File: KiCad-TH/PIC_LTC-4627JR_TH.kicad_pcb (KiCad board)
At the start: 2 copper layers, 43.2 x 48.3 mm, 17 parts, among them J1 Conn_01x05_Male, J2 Conn_01x04, Q1 Q_NPN_EBC, Q2 Q_NPN_EBC, Q3 Q_NPN_EBC, Q4 Q_NPN_EBC, Q5 Q_NPN_EBC, U1 PIC16F18344-P

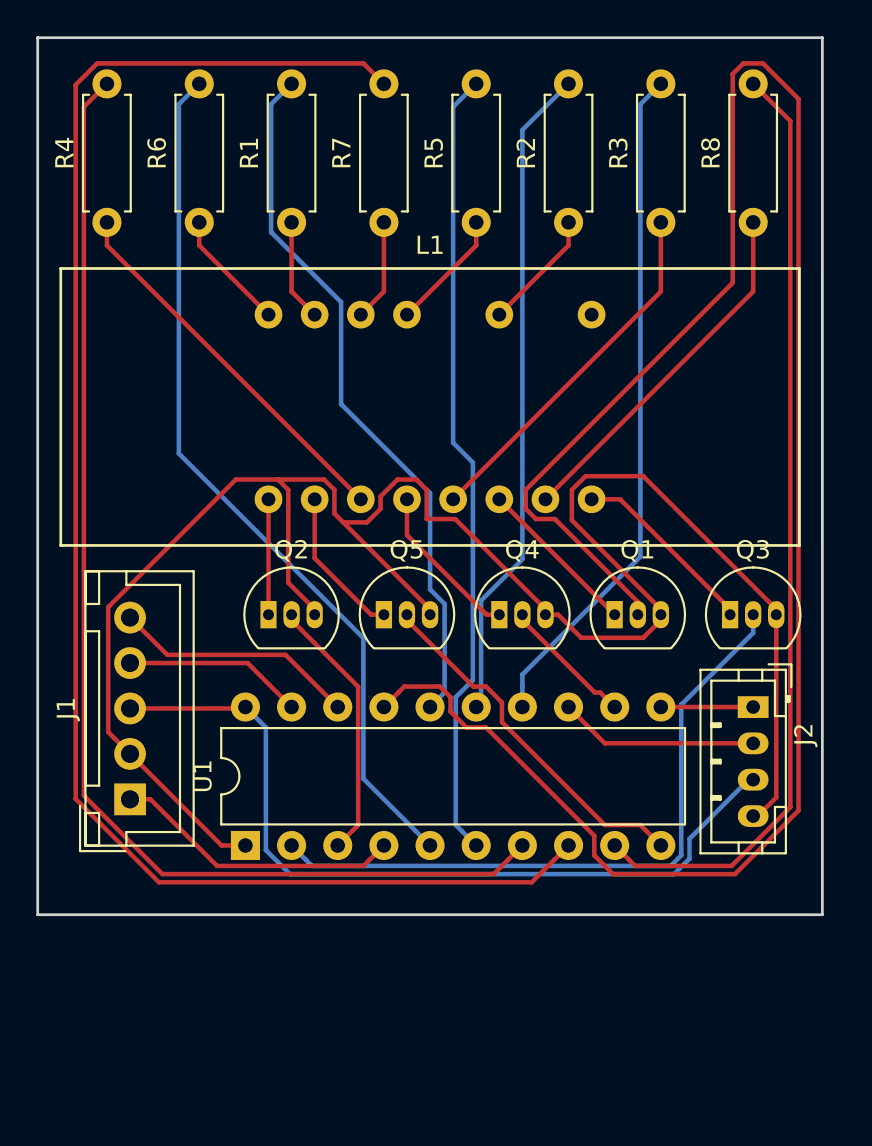
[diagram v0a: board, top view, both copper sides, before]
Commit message: PCB Routing Round #3: Getting better, still room for improvement.
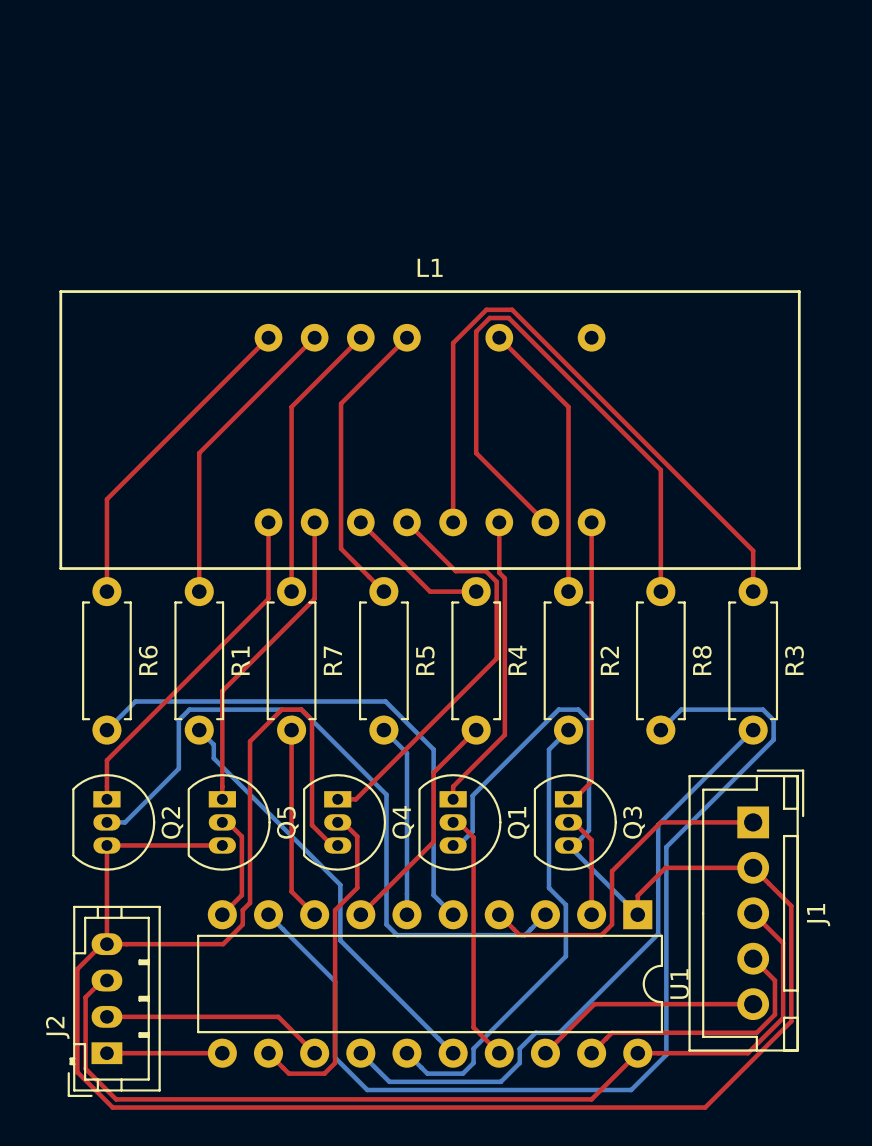
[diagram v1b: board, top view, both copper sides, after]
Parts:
- moved J2 40.3 mm to (111.8, 128.3), turned to 90 degrees
- moved J1 34.3 mm to (147.3, 115.6), turned to 270 degrees
- moved R4 28.7 mm to (132.1, 102.9), turned to 270 degrees
- moved U1 21.9 mm to (141.0, 120.7), turned to 270 degrees
- moved R1 20.9 mm to (116.8, 102.9), turned to 270 degrees
- moved R5 20.9 mm to (127.0, 102.9), turned to 270 degrees
- moved R6 20.9 mm to (111.8, 102.9), turned to 270 degrees
- moved R7 20.9 mm to (121.9, 102.9), turned to 270 degrees
- moved R3 20.9 mm to (147.3, 102.9), turned to 270 degrees
- moved R8 20.9 mm to (142.2, 102.9), turned to 270 degrees
- moved R2 20.3 mm to (137.2, 102.9), turned to 270 degrees
- moved Q3 13.5 mm to (137.2, 114.3), turned to 270 degrees
- moved Q2 13.5 mm to (111.8, 114.3), turned to 270 degrees
- moved Q4 13.5 mm to (124.5, 114.3), turned to 270 degrees
- moved Q5 13.5 mm to (118.1, 114.3), turned to 270 degrees
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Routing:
- net Net-(Q1-Pad2): track 111.6 -> 13.9 mm
- net Net-(R7-Pad2): track 87.1 -> 10.7 mm
- net Net-(R4-Pad2): track 66.3 -> 12.8 mm
- net Net-(R5-Pad2): track 43.7 -> 10.7 mm
- net Net-(Q3-Pad2): track 37.0 -> 5.78 mm
- net VCC: track 109.7 -> 134.1 mm
- net Net-(Q2-Pad2): track 14.7 -> 38.1 mm
- net Net-(R6-Pad2): track 48.1 -> 29.3 mm
- net Net-(R1-Pad2): track 39.0 -> 23.6 mm
- net Net-(L1-Pad5): track 20.0 -> 34.9 mm
- net Net-(Q5-Pad2): track 20.0 -> 6.15 mm
- net /DIG_L: track 8.86 -> 22.5 mm
- net Net-(L1-Pad3): track 21.0 -> 7.93 mm
- net Net-(L1-Pad7): track 20.0 -> 32.7 mm
- net /DIG_1: track 6.35 -> 18.9 mm
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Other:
- board outline removed
